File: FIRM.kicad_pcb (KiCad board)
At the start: 8 copper layers, 21.3 x 27 mm, 97 parts, among them J1 DM3CS-SF, J2 Conn_01x02_Pin, Q1 IRLML6402, U1 W25Q128JVP, U2 STM32F405RGTx, U3 ADXL371, U5 INA219AxDCN, U6 MIC5219-3.3YM5, U9 A-USBC-20F0-EA-GSR05, X1 32.768khz, Y1 12 MHz

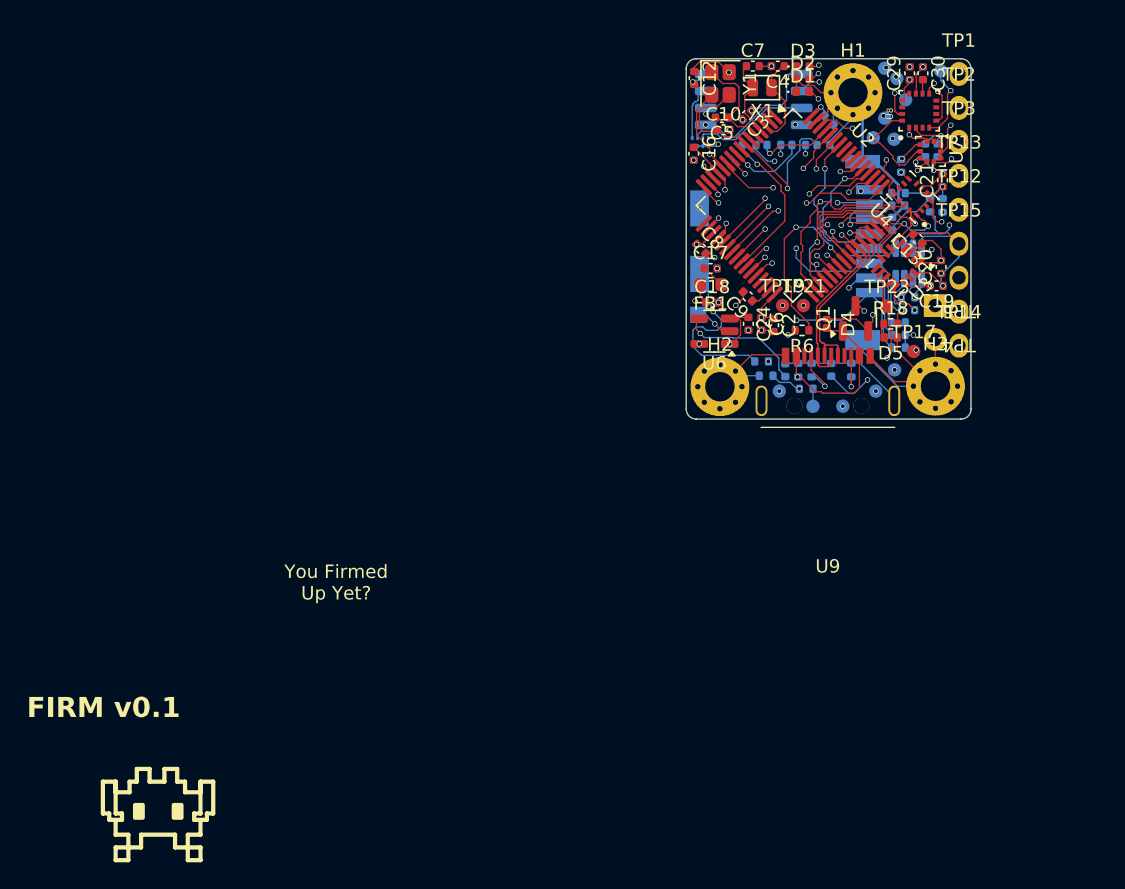
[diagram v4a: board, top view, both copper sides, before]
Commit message: silkscreen
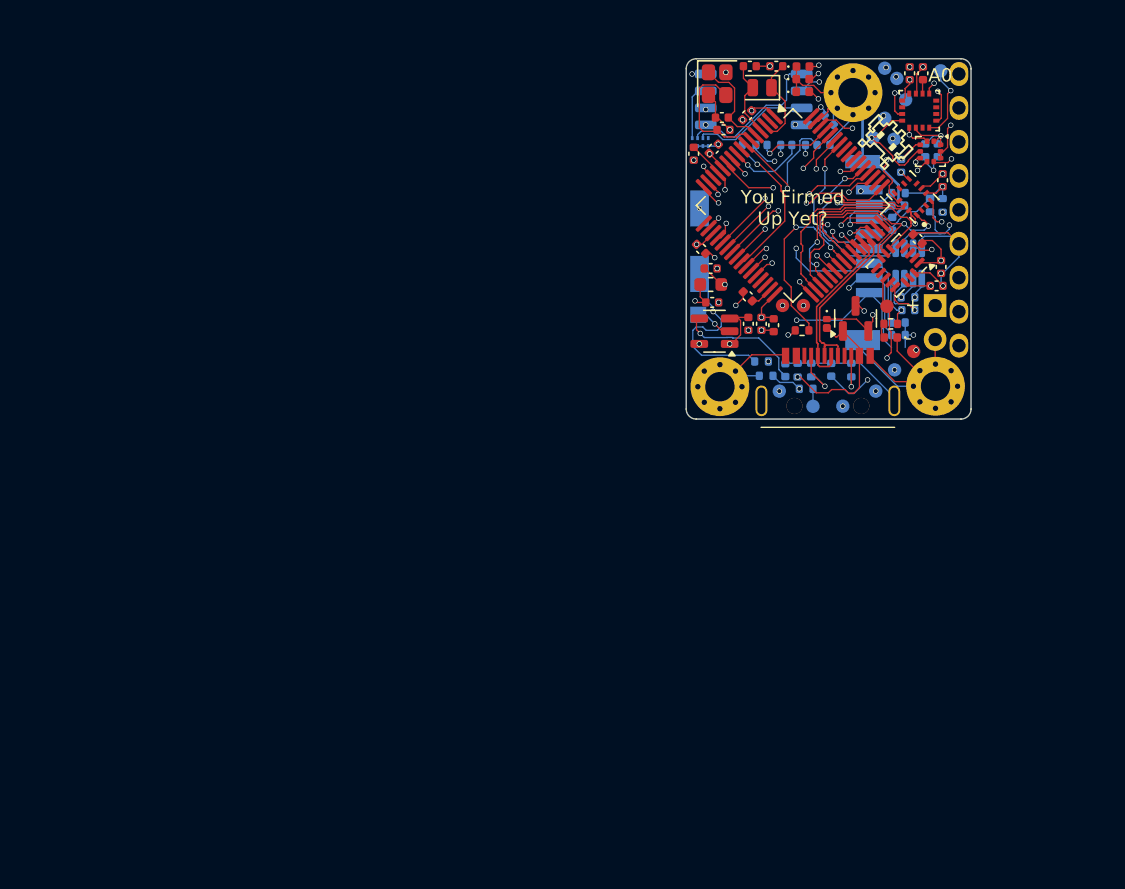
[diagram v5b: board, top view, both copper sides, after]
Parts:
- removed R1: 47k, Resistor_SMD:R_0402_1005Metric
- added G***: LOGO, connectors:firm-logo, F.Cu at (168.2, 80.8)
- moved C12 5.49 mm to (155.4, 81.3), turned to 45 degrees
- moved Y1 0.25 mm to (155.7, 76.4)
- moved C7 0.23 mm to (158.1, 75.1)
- moved C4 0.12 mm to (160.1, 75.1)
- renumbered TP1 to A0, TP2 to A1, TP17 to BMP_CS, TP15 to GD, TP16 to IMU, TP18 to MAG, TP8 to SPI, TP13 to SWCLK, TP6 to a4
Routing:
- net GND: track 117.4 -> 110.1 mm
- net /SCK2: track 44.8 -> 51.2 mm
- net /PA9: track 16.4 -> 15.1 mm
- net /HSE_OUT: track 7.71 -> 9.08 mm
- net VBUS: track 13.0 -> 11.9 mm
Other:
- board text added: "+"
- board text added: "-"
- board text added: "I2C"
- board text removed: "FIRM v0.1"
